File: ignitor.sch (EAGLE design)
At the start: 80 parts, among them IC1 T2333, IC2 TA80005, IC3 D131850-0760, T1 B647, T2 C945, T3 1005, T4 MJE801, T5 1005, T6 MJE801, U1 ATMEGA48-20PU, X1 12.07 MHz

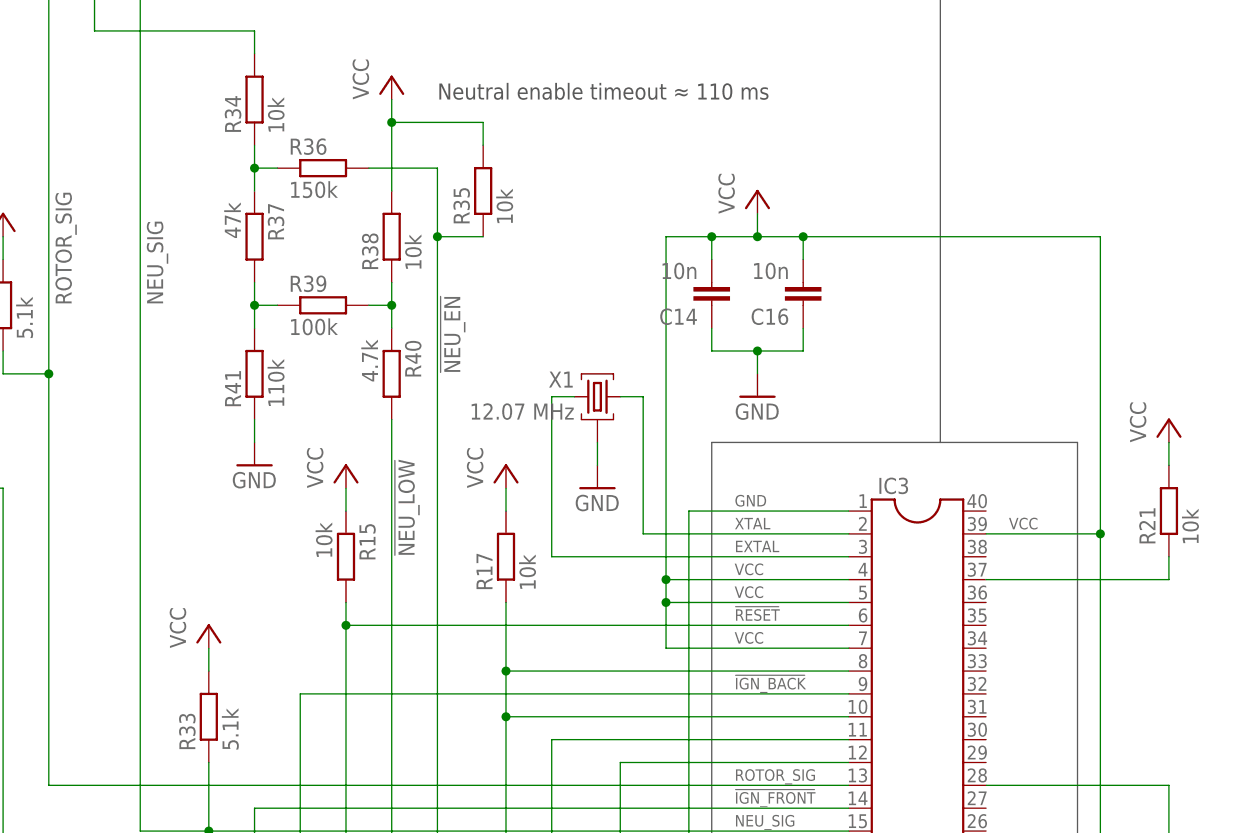
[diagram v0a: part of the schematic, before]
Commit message: Memory keep
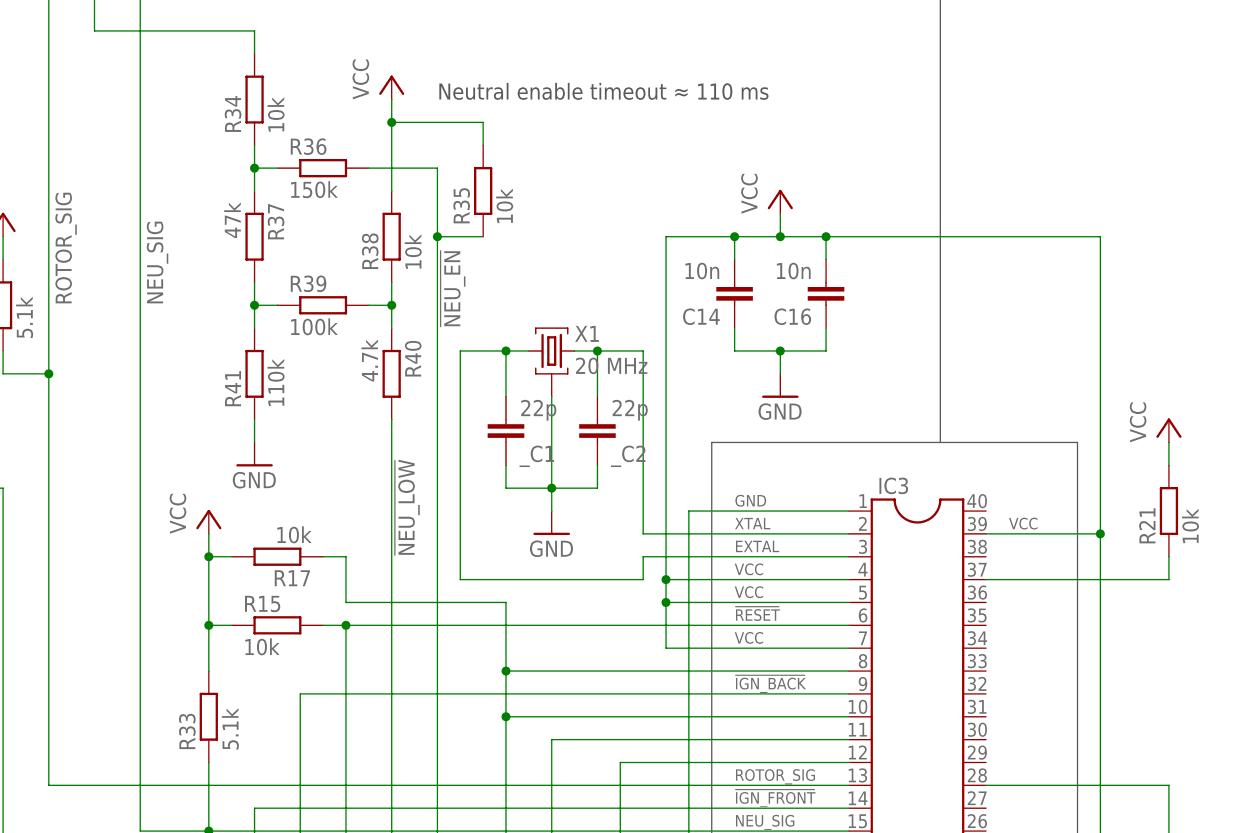
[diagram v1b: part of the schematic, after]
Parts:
- added _C1, _C2: 22p, resistor:C-EUC0805
- X1: value 12.07 MHz -> 20 MHz
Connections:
- net EXTAL: now also X1.1, _C1.2; no longer X1.3
- net GND: now also _C1.1, _C2.1
- net XTAL: now also X1.3, _C2.2; no longer X1.1
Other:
- moved on the sheet: C14, C16, R15, R17, X1
